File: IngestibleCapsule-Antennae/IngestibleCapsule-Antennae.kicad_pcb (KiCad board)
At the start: 2 copper layers, 58.6 x 27 mm, 5 parts, among them J1 BM02B, J2 BM02B, U1 HHM1595A1

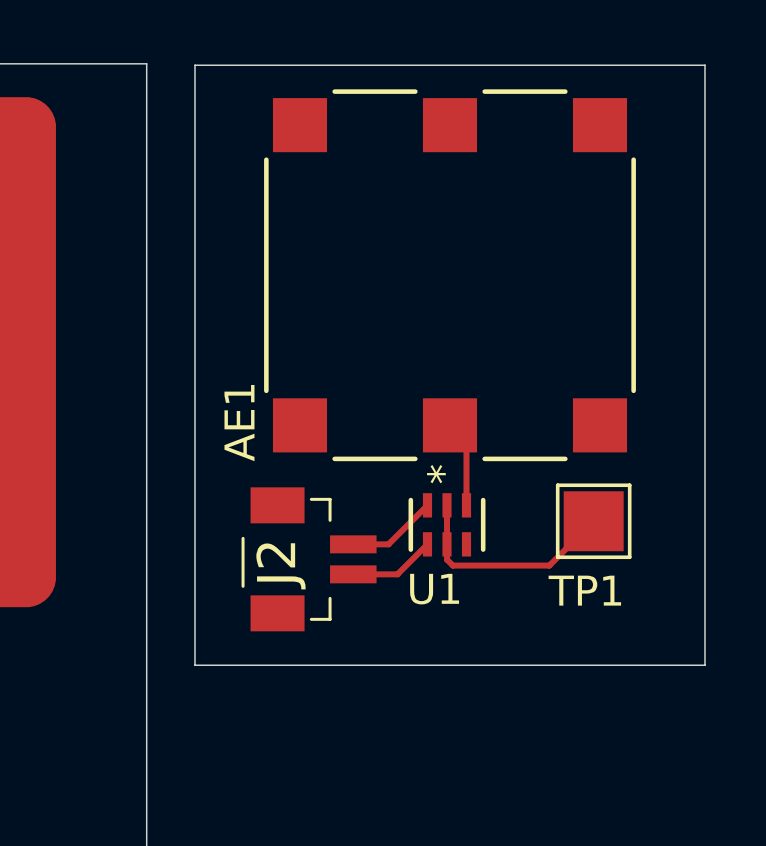
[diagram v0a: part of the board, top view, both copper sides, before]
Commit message: beginning a whole board
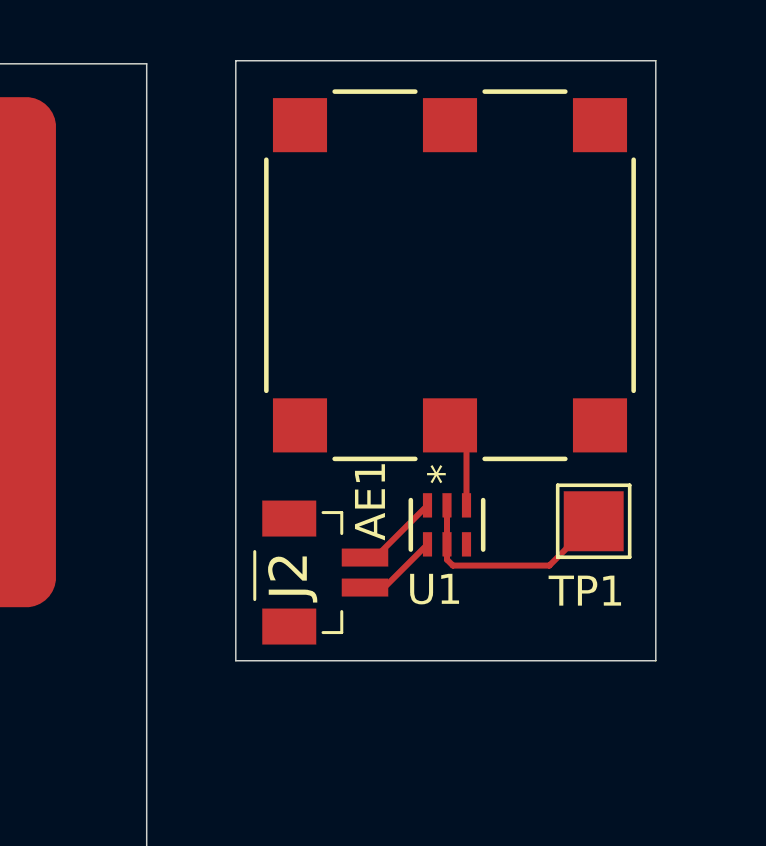
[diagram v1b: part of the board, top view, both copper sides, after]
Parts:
- moved J2 0.59 mm to (75.4, 55.2)
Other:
- board size 58.6 x 27 mm -> 57 x 27.1 mm
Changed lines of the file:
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@@
 			(drillshape 0)
 			(scaleselection 1)
-			(outputdirectory "Gerbers-Antennae/")
+			(outputdirectory "Gerbers-SMD/")
 		)
 	)
@@
 	(footprint "kjp_fplib:BM02BSRSSTBLFSN"
 		(layer "F.Cu")
-		(at 75.05 54.78 -90)
+		(at 75.44 55.22 -90)
 		(descr "BM02B-SRSS-TB(LF)(SN)-3")
 		(tags "Connector")
@@
 		(tags "UWC.20 ")
 		(property "Reference" "AE1"
-			(at -4.87 -6.98 90)
+			(at -7.51 -2.63 90)
 			(unlocked yes)
 			(layer "F.SilkS")
@@
 	)
 	(gr_rect
-		(start 71.61 38.31)
-		(end 88.61 58.31)
+		(start 72.97 38.16)
+		(end 86.97 58.16)
 		(stroke
 			(width 0.05)
@@
 	)
 	(segment
-		(start 78.360002 55.28)
+		(start 77.277 55.72)
+		(end 77.920002 55.72)
+		(width 0.2)
+		(layer "F.Cu")
+		(net 3)
+	)
+	(segment
+		(start 77.920002 55.72)
 		(end 79.360002 54.28)
 		(width 0.2)
@@
 	)
 	(segment
-		(start 76.887 55.28)
-		(end 78.360002 55.28)
-		(width 0.2)
-		(layer "F.Cu")
-		(net 3)
-	)
-	(segment
-		(start 76.887 54.28)
-		(end 78.060004 54.28)
-		(width 0.2)
-		(layer "F.Cu")
-		(net 4)
-	)
-	(segment
-		(start 78.060004 54.28)
+		(start 77.620004 54.72)
 		(end 79.360002 52.980002)
 		(width 0.2)
 		(layer "F.Cu")
+		(net 4)
+	)
+	(segment
+		(start 77.277 54.72)
+		(end 77.620004 54.72)
+		(width 0.2)
+		(layer "F.Cu")
